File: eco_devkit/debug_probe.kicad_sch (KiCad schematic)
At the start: 26 parts, among them J1 Conn_01x06_Pin, J2 USB_C_Receptacle_USB2.0_16P, Y1 ABM8-272-T3

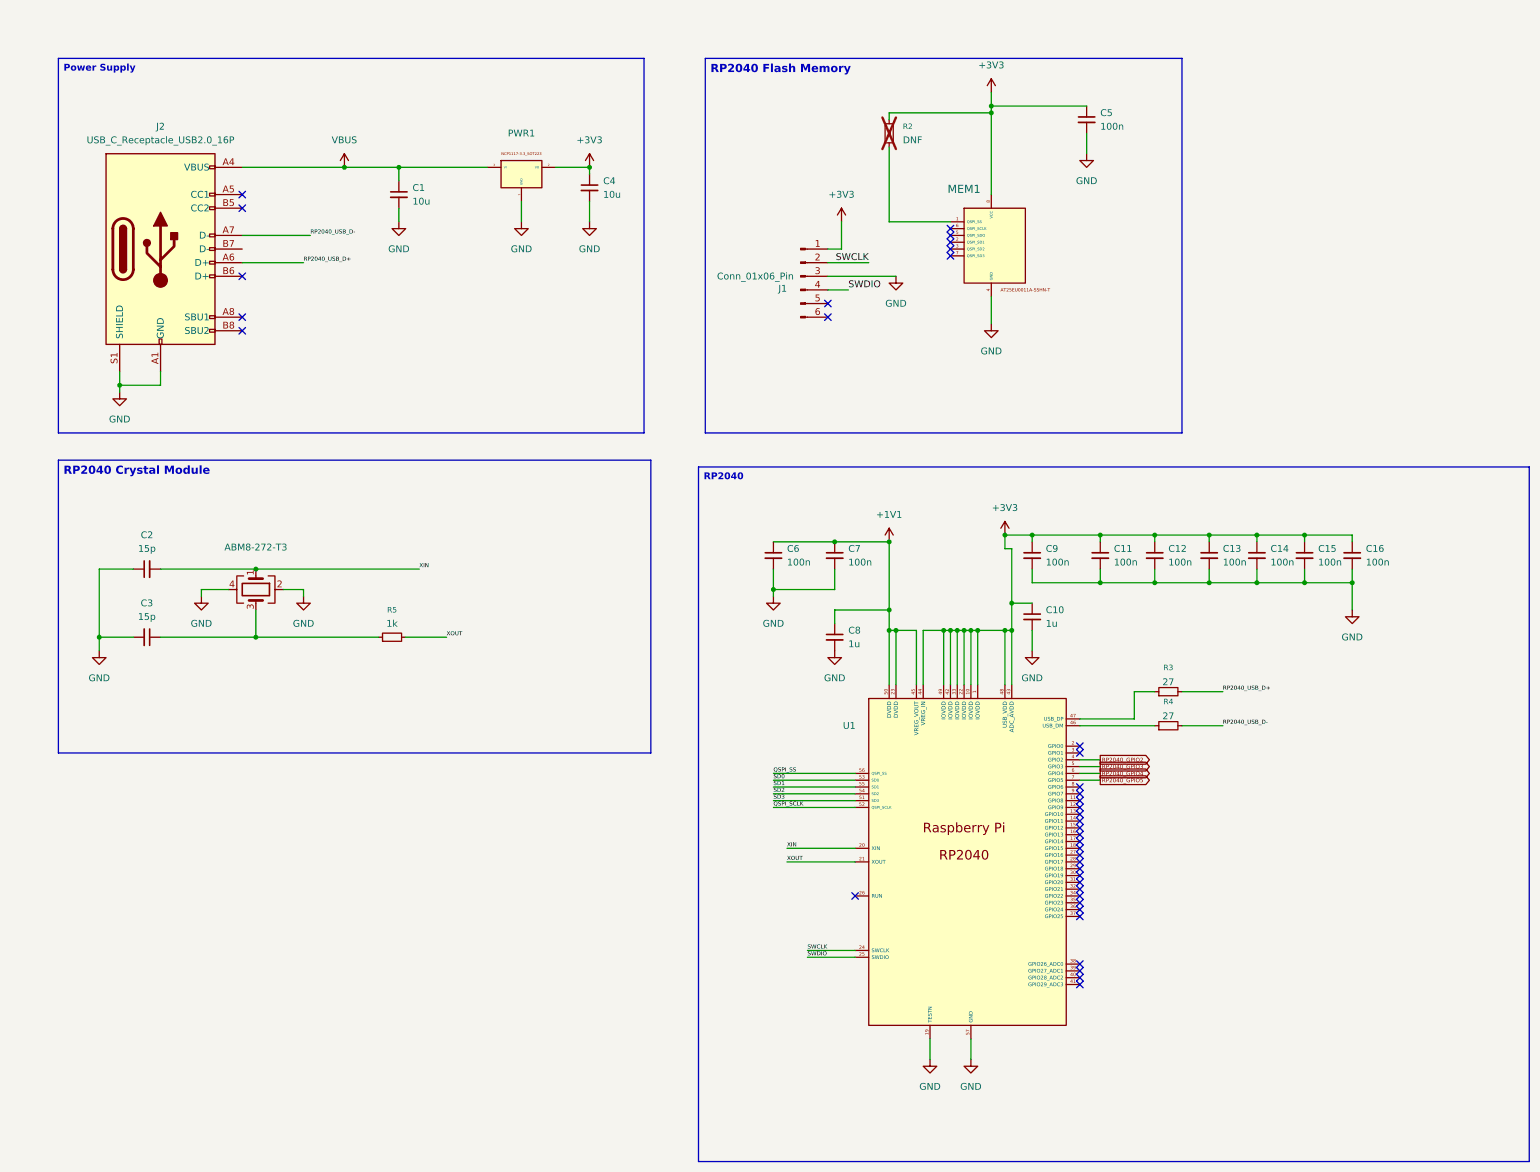
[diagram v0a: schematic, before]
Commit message: Update layout
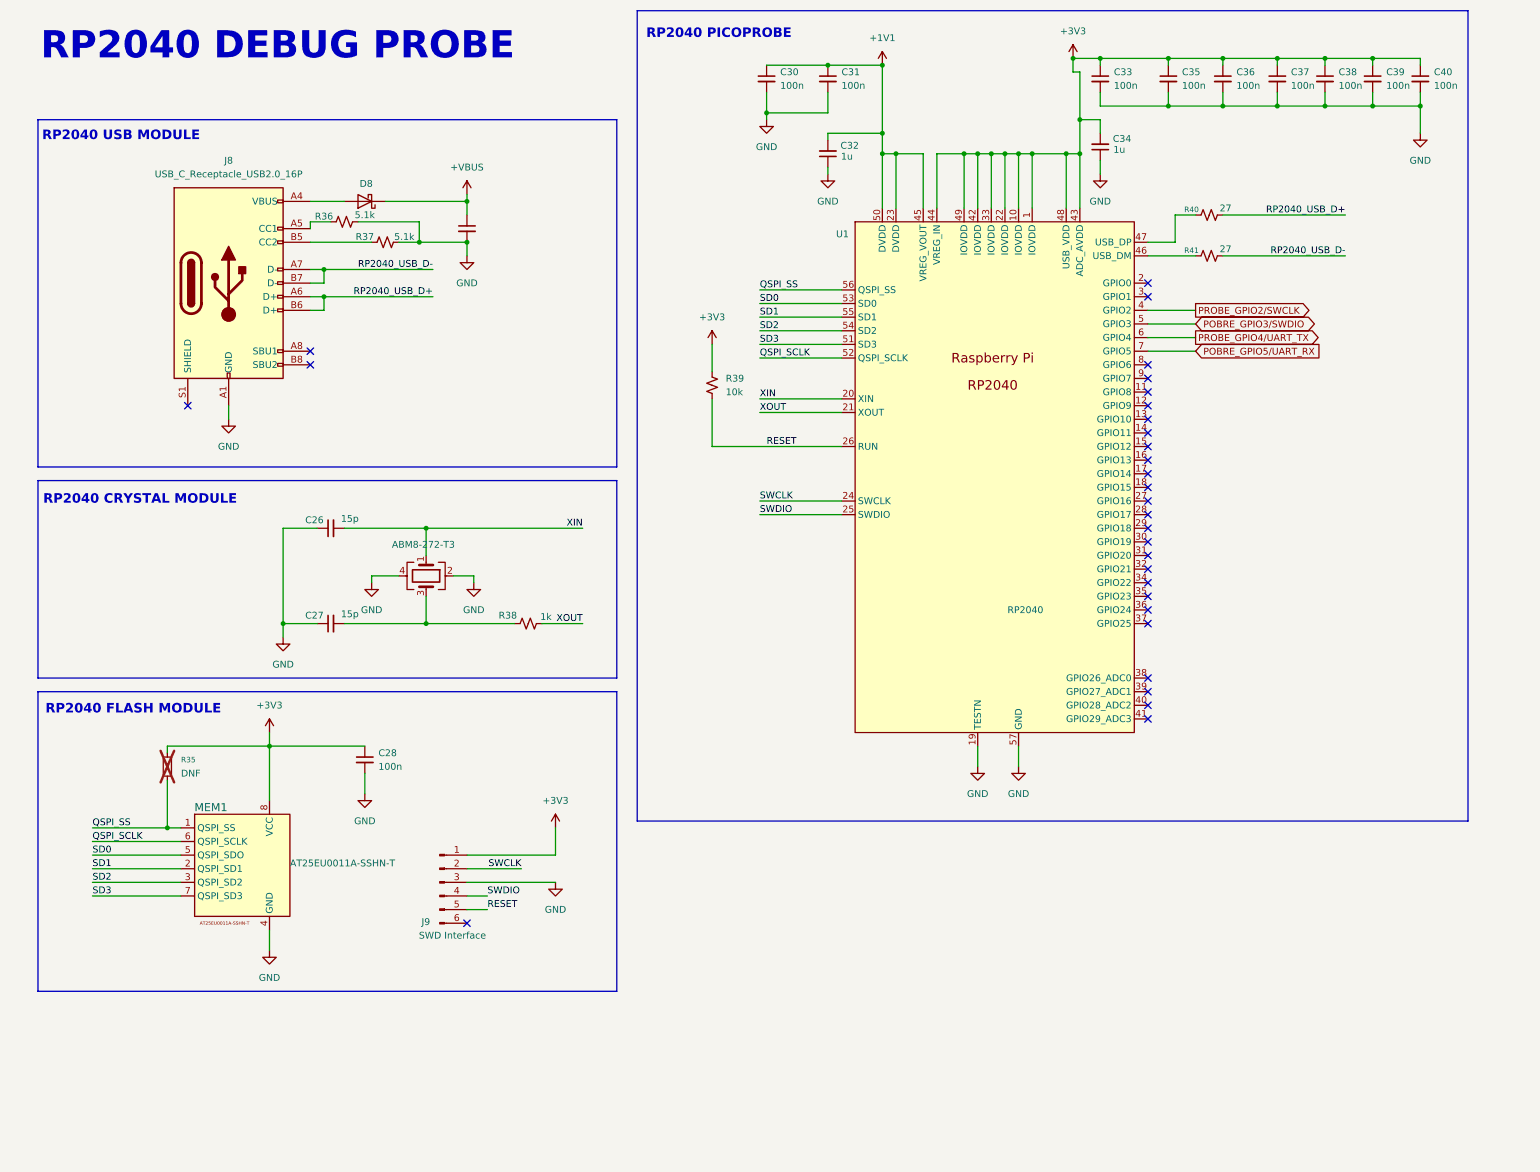
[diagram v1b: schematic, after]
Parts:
- removed C1, C4: 10u, Capacitor_SMD:C_0402_1005Metric, symbol Device:C_Small
- removed C10, C8: 1u, Capacitor_SMD:C_0402_1005Metric, symbol Device:C_Small
- removed C11, C12, C13, C14, C15, C16, C5, C6, C7, C9: 100n, Capacitor_SMD:C_0402_1005Metric, symbol Device:C_Small
- removed C3: 15p, Capacitor_SMD:C_0402_1005Metric, symbol Device:C_Small
- removed J2: USB_C_Receptacle_USB2.0_16P, Connector_USB:USB_C_Receptacle_HCTL_HC-TYPE-C-16P-01A, symbol Connector:USB_C_Receptacle_USB2.0_16P
- removed PWR1: ~, Footprint-NP1117-POWER-SUPPLY:SOT230P700X175-4N, symbol PROBE-SYMBOL-LIB:NCP1117-3.3SOT_223
- removed R4: 27, Resistor_SMD:R_0402_1005Metric, symbol Device:R_Small
- removed R5: 1k, Resistor_SMD:R_0402_1005Metric, symbol Device:R_Small
- added C27: 15p, Capacitor_SMD:C_0603_1608Metric, symbol Device:C_Small
- added C28, C30, C31, C33, C35, C36, C37, C38, C39, C40: 100n, Capacitor_SMD:C_0402_1005Metric, symbol Device:C_Small
- added C29: 10u, Capacitor_SMD:C_0402_1005Metric, symbol Device:C_Small
- added C32, C34: 1u, Capacitor_SMD:C_0402_1005Metric, symbol Device:C_Small
- added D8: SB120, Diode_SMD:D_SOD-123F, symbol Diode:SB120
- added J8: USB_C_Receptacle_USB2.0_16P, lib:UJ20-C-H-G-SMT-1-P16-TR, symbol Connector:USB_C_Receptacle_USB2.0_16P
- added R36, R37: 5.1k, Resistor_SMD:R_0402_1005Metric, symbol Device:R_Small_US
- added R38: 1k, Resistor_SMD:R_0402_1005Metric, symbol Device:R_Small_US
- added R39: 10k, Resistor_SMD:R_0402_1005Metric, symbol Device:R_Small_US
- added R41: 27, Resistor_SMD:R_0402_1005Metric, symbol Device:R_Small_US
- C26: renamed from C2; footprint Capacitor_SMD:C_0402_1005Metric -> Capacitor_SMD:C_0603_1608Metric; MPN (none) -> C0603C150K8RACAUTO
- J9: renamed from J1; value Conn_01x06_Pin -> SWD Interface
- MEM1: value ~ -> AT25EU0011A-SSHN-T; MPN (none) -> AT25EU0011A-SSHN-T
- R40: renamed from R3; symbol Device:R_Small -> Device:R_Small_US; MPN (none) -> RCS040227R0FKED
- U1: value ~ -> RP2040
- Y2: renamed from Y1; footprint ABM8_272_T3:XTAL_ABM8-272-T3 -> lib:ABM8-272-T3; MPN (none) -> ABM8-272-T3
- renumbered R2 to R35
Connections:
- net +1V1: now also C30.1, C31.1, C32.2
- net +3V3: now also C28.1, C33.1, C34.2, C35.1, C36.1, C37.1, C38.1, C39.1, C40.1, R39.1
- net GND: now also C27.1, C28.2, C29.2, C30.2, C31.2, C32.1, C33.2, C34.1, C35.2, C36.2, C37.2, C38.2, C39.2, C40.2, J8.A1 (GND), J8.A12 (GND), J8.B1 (GND), J8.B12 (GND), R36.2, R37.2
- net QSPI_SCLK: now also MEM1.6 (QSPI_SCLK)
- net QSPI_SS: now also MEM1.1 (QSPI_SS), R35.1
- net RP2040_USB_D+: now also J8.A6 (D+), J8.B6 (D+)
- net RP2040_USB_D-: now also J8.A7 (D-), J8.B7 (D-), R41.2
- net SD0: now also MEM1.5 (QSPI_SDO)
- net SD1: now also MEM1.2 (QSPI_SD1)
- net SD2: now also MEM1.3 (QSPI_SD2)
- net SD3: now also MEM1.7 (QSPI_SD3)
- net XOUT: now also R38.2
- net RESET: now reaches J9.5 (Pin_5)
- net RESET: now also U1.26 (RUN), R39.2
- net at Y2.3: now also C27.2, R38.1
- net at U1.46 (USB_DM): now also R41.1
- net RP2040_GPIO2 renamed PROBE_GPIO2/SWCLK
- net RP2040_GPIO3 renamed POBRE_GPIO3/SWDIO
- net RP2040_GPIO4 renamed PROBE_GPIO4/UART_TX
- net RP2040_GPIO5 renamed POBRE_GPIO5/UART_RX
- new net: J8.A5 (CC1), R36.1
- new net: J8.B5 (CC2), R37.1
- new net: D8.2 (A), J8.A4 (VBUS), J8.A9 (VBUS), J8.B4 (VBUS), J8.B9 (VBUS)
- new net +VBUS: C29.1, D8.1 (K)
- no-connect marks 39 -> 30
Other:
- note added: "RP2040 CRYSTAL MODULE"
- note added: "RP2040 DEBUG PROBE"
- note added: "RP2040 FLASH MODULE"
- note added: "RP2040 PICOPROBE"
- note added: "RP2040 USB MODULE"
- moved on the sheet: C26, J9, MEM1, R35
